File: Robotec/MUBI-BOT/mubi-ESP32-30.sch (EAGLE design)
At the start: 37 parts, among them IC1 L293D, IC2 7805T

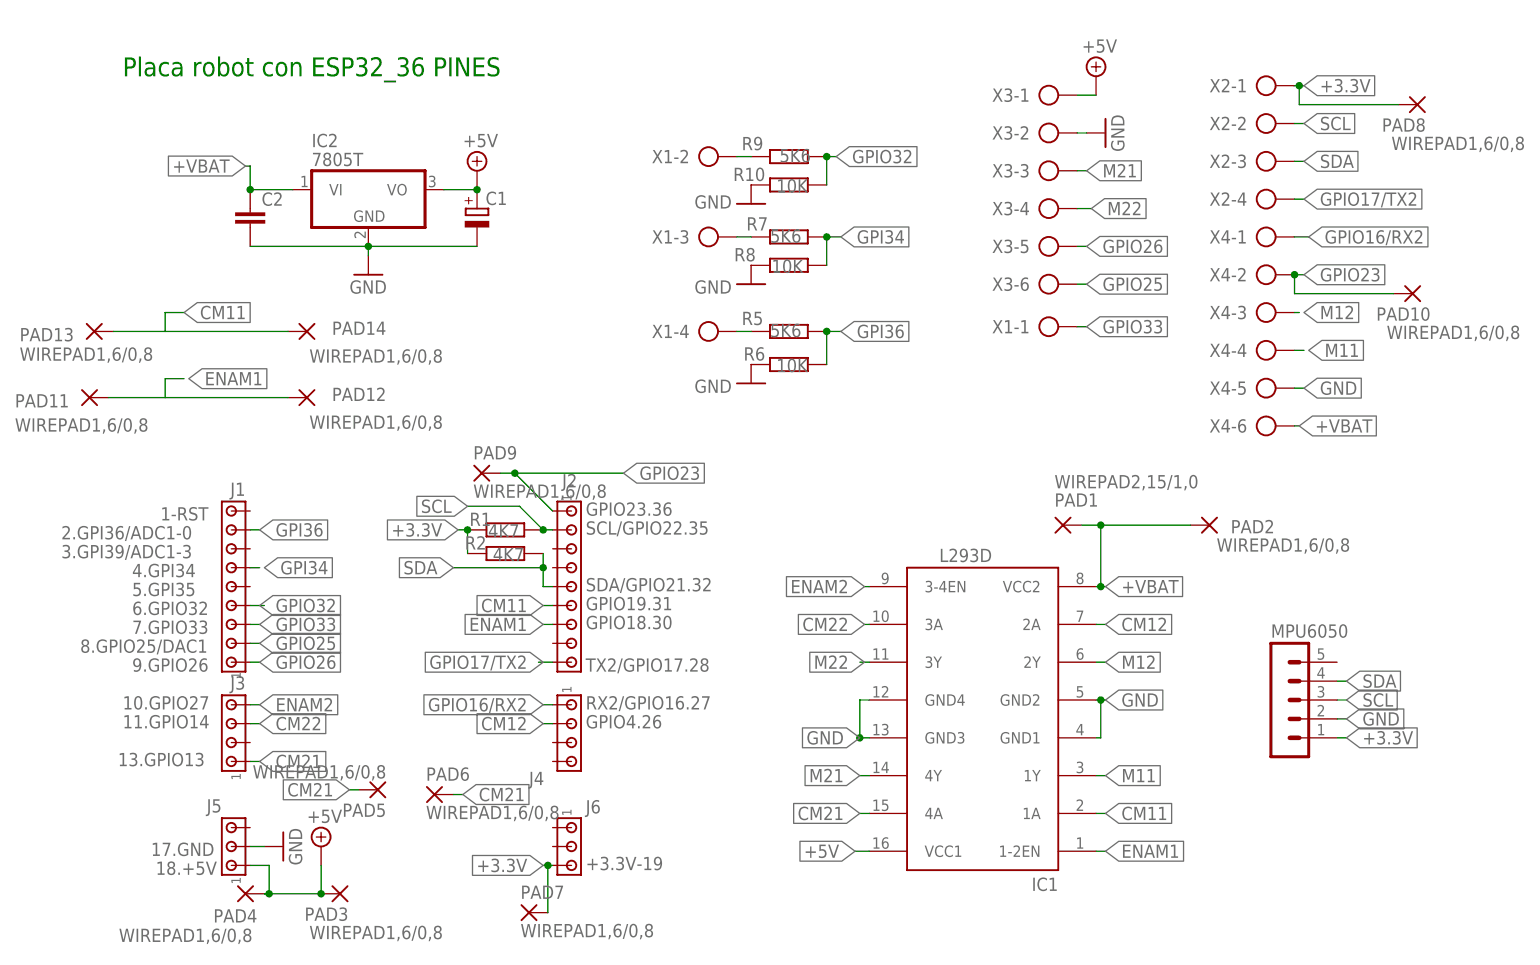
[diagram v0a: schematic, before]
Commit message: update sch & brd
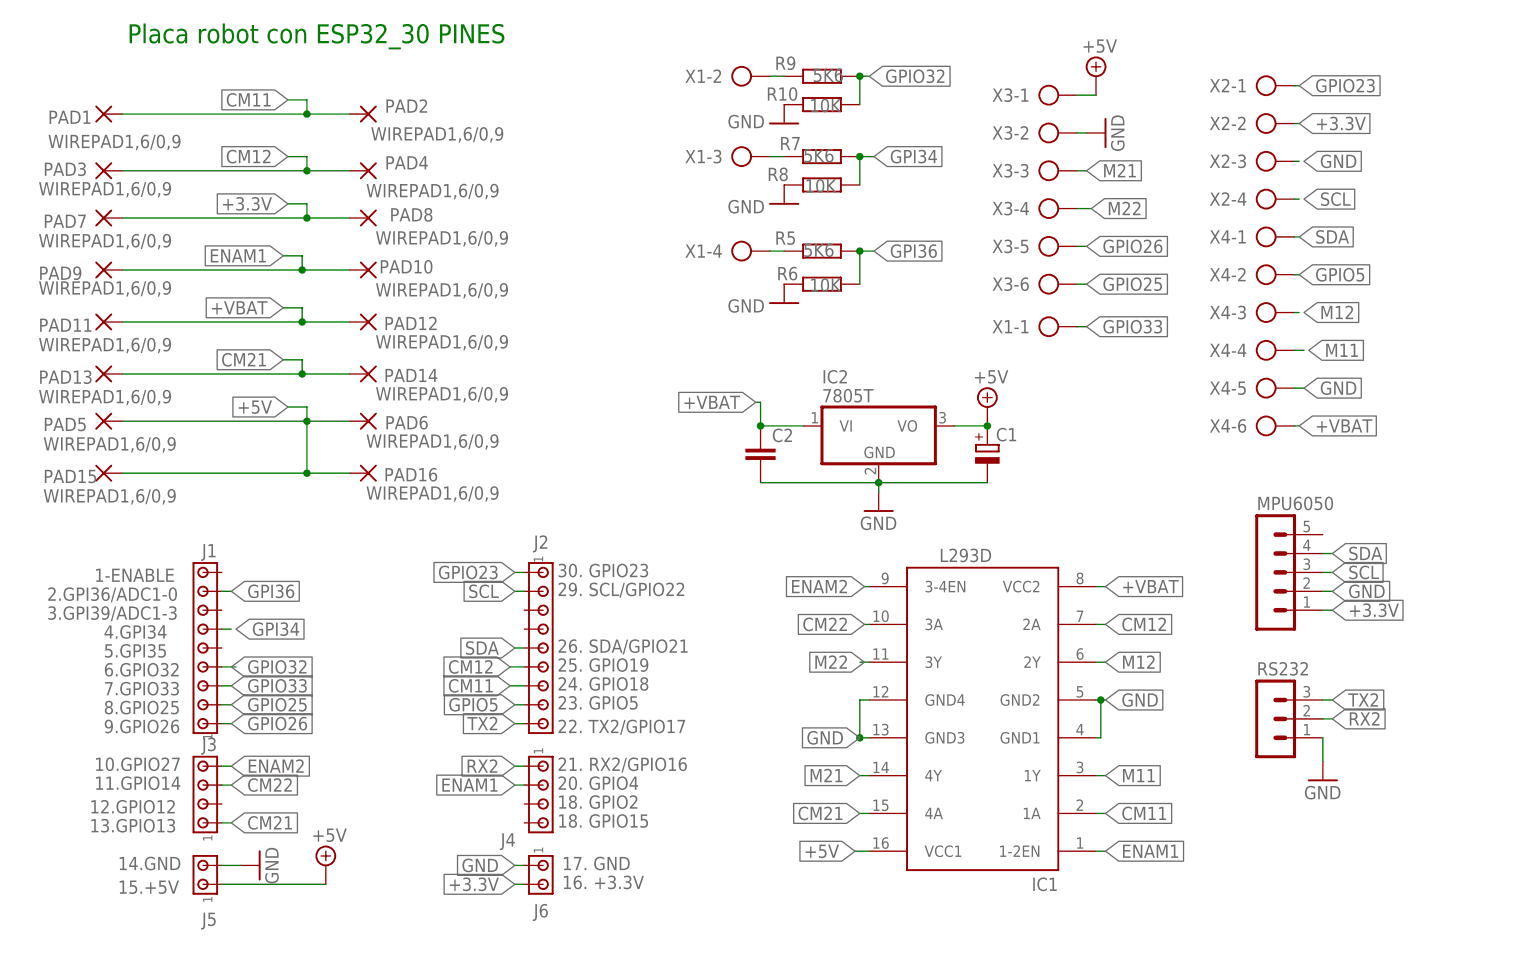
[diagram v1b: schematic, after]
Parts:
- removed R1, R2: 4K7, rcl:R-EU_0207/7
- added PAD15, PAD16: WIREPAD1,6/0,9, wirepad:WIREPAD1,6/0,9
- added RS232: (no value), con-lstb:MA03-1
- J5, J6: device con-amp:MTA03-100 -> con-amp:MTA02-100
- PAD1: value WIREPAD2,15/1,0 -> WIREPAD1,6/0,9; device wirepad:WIREPAD2,15/1,0 -> wirepad:WIREPAD1,6/0,9
- PAD10, PAD11, PAD12, PAD13, PAD14, PAD2, PAD3, PAD4, PAD5, PAD6, PAD7, PAD8, PAD9: value WIREPAD1,6/0,8 -> WIREPAD1,6/0,9; device wirepad:WIREPAD1,6/0,8 -> wirepad:WIREPAD1,6/0,9
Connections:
- removed net GPIO16/RX2: J4.1, X4-1.KL
- removed net GPIO17/TX2: J2.9, X2-4.KL
- new net GPIO5: J2.8, X4-2.KL
- new net RX2: J4.1, RS232.2
- new net TX2: J2.9, RS232.3
- net +3.3V: now also J6.2, X2-2.KL; no longer J6.3, R1.2, R2.2, X2-1.KL
- net +5V: now also PAD15.P, PAD16.P, PAD5.P, PAD6.P; no longer PAD3.P, PAD4.P
- net +VBAT: now also PAD11.P, PAD12.P; no longer PAD1.P, PAD2.P
- net CM11: now also J2.7, PAD1.P, PAD2.P; no longer J2.6, PAD13.P, PAD14.P
- net CM12: now also J2.6, PAD3.P, PAD4.P; no longer J4.2
- net CM21: now also PAD13.P, PAD14.P; no longer PAD5.P, PAD6.P
- net ENAM1: now also J4.2, PAD10.P, PAD9.P; no longer J2.7, PAD11.P, PAD12.P
- net GND: now also J6.1, RS232.1, X2-3.KL
- net GPIO23: now also X2-1.KL; no longer PAD10.P, PAD9.P, X4-2.KL
- net SCL: now also X2-4.KL; no longer R1.1, X2-2.KL
- net SDA: now also X4-1.KL; no longer R2.1, X2-3.KL
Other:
- note added: "1-ENABLE"
- note added: "12.GPIO12"
- note added: "14.GND"
- note added: "15.+5V"
- note added: "16. +3.3V"
- note added: "17. GND"
- note added: "18. GPIO15"
- note added: "18. GPIO2"
- note added: "20. GPIO4"
- note added: "21. RX2/GPIO16"
- note added: "22. TX2/GPIO17"
- note added: "23. GPIO5"
- note added: "24. GPIO18"
- note added: "25. GPIO19"
- note added: "26. SDA/GPIO21"
- note added: "29. SCL/GPIO22"
- note added: "30. GPIO23"
- note added: "8.GPIO25"
- note added: "Placa robot con ESP32_30 PINES"
- note removed: "+3.3V-19"
- note removed: "1-RST"
- note removed: "17.GND"
- note removed: "18.+5V"
- note removed: "8.GPIO25/DAC1"
- note removed: "GPIO18.30"
- note removed: "GPIO19.31"
- note removed: "GPIO23.36"
- note removed: "GPIO4.26"
- note removed: "Placa robot con ESP32_36 PINES"
- note removed: "RX2/GPIO16.27"
- note removed: "SCL/GPIO22.35"
- note removed: "SDA/GPIO21.32"
- note removed: "TX2/GPIO17.28"
- moved on the sheet: C1, C2, IC2, J1, J2, J3, J4, MPU6050, PAD1, PAD10, PAD11, PAD12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
